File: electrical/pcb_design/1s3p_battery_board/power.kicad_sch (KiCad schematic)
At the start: 11 parts, among them U8 TPS63900

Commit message: Move 1s3p battery board to KiCad 9
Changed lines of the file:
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@@
 (kicad_sch
-	(version 20231120)
+	(version 20250114)
 	(generator "eeschema")
-	(generator_version "8.0")
+	(generator_version "9.0")
 	(paper "USLetter")
 	(title_block
@@
 		)
 		(instances
-			(project ""
+			(project "1s3p_battery_board"
 				(path "/695f882b-5312-4493-b26d-8f7d6768a9db/7f8fc7f5-7f1e-476b-9e93-5575de1d6778"
 					(reference "L1")
@@
 		)
 		(instances
-			(project ""
+			(project "1s3p_battery_board"
 				(path "/695f882b-5312-4493-b26d-8f7d6768a9db/7f8fc7f5-7f1e-476b-9e93-5575de1d6778"
 					(reference "U8")

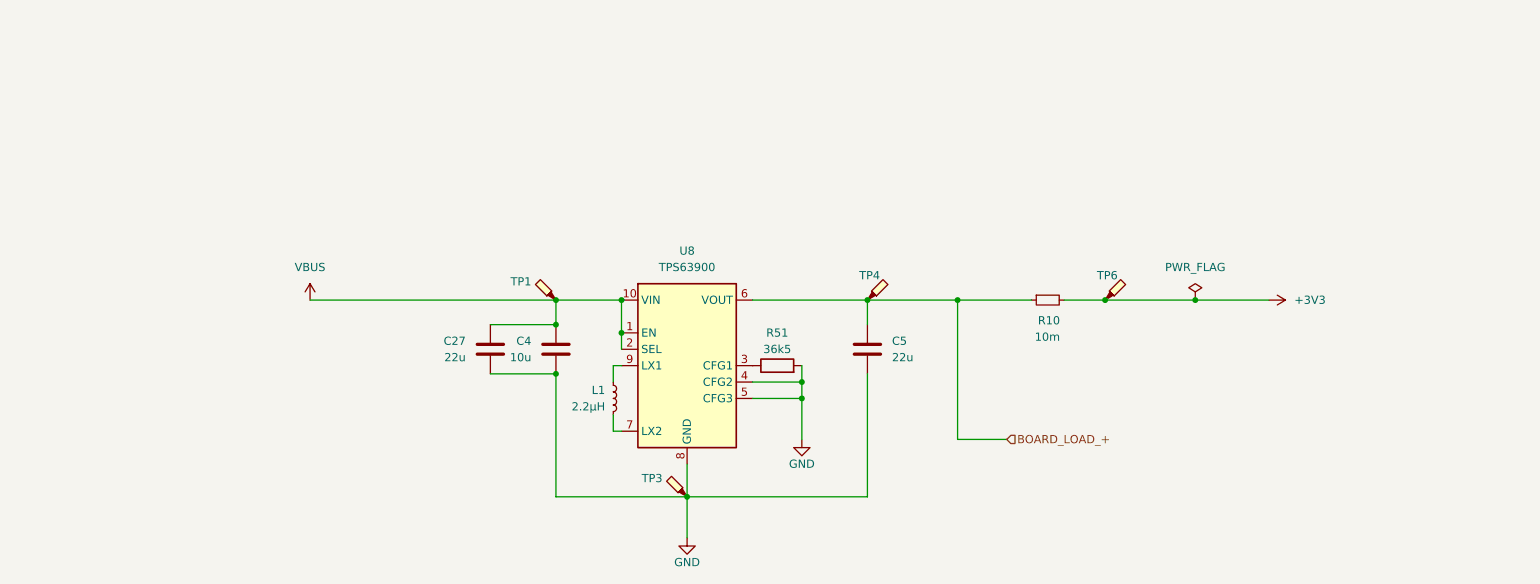
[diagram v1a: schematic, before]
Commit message: Checkpoint work on 1s3p battery board
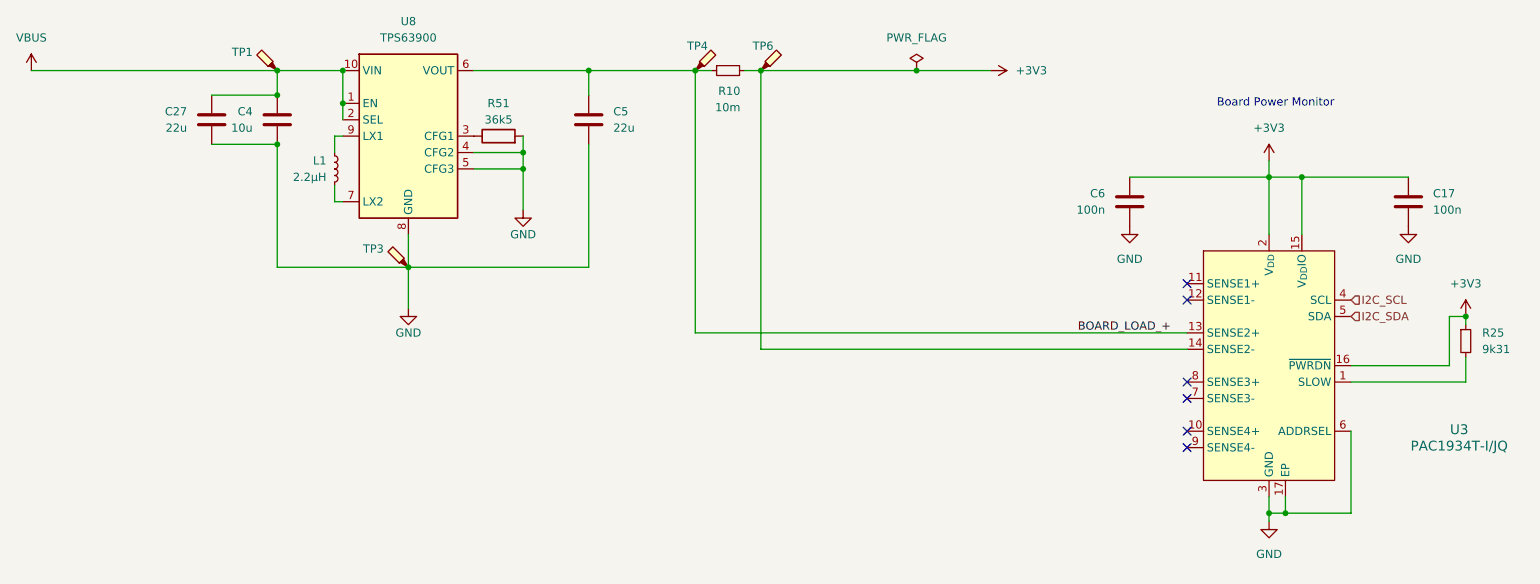
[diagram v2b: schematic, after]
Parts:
- added C17, C6: 100n, footprints:Nondescript_C_0402_1005Metric, symbol Device:C
- added R25: 9k31, footprints:Nondescript_R_0402_1005Metric, symbol Device:R_Small
- added U3: PAC1934T-I/JQ, footprints:UQFN-16-1EP_4x4mm_P0.65mm_EP2.6x2.6mm, symbol Sensor_Energy:PAC1934x-xJQ
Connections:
- net +3V3: now also C17.1, C6.1, R25.1, U3.14 (SENSE2-), U3.15 (V_{DD}IO), U3.16 (~{PWRDN}), U3.2 (V_{DD})
- net BOARD_LOAD_+: now also U3.13 (SENSE2+)
- net GND: now also C17.2, C6.2, U3.17 (EP), U3.3 (GND), U3.6 (ADDRSEL)
- new net: R25.2, U3.1 (SLOW)
- new net I2C_SCL: U3.4 (SCL)
- new net I2C_SDA: U3.5 (SDA)
- no-connect marks 0 -> 6
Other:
- note added: "Board Power Monitor"
- moved on the sheet: C27, C4, C5, L1, R10, R51, TP1, TP3, TP4, TP6, U8
